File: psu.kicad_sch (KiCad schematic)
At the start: 63 parts, among them J3 USB_C_Receptacle_PowerOnly_24P, J4 Screw_Terminal_01x02, J5 Screw_Terminal_01x02, J6 Screw_Terminal_01x03, Q1 2N7002, Q2 DMP3099L, Q3 DMP3099L, U17 CYPD3177-24LQ, U19 LM2596S-ADJ, U20 INA180A3, U21 LM2596S-5, U22 LM2596S-5

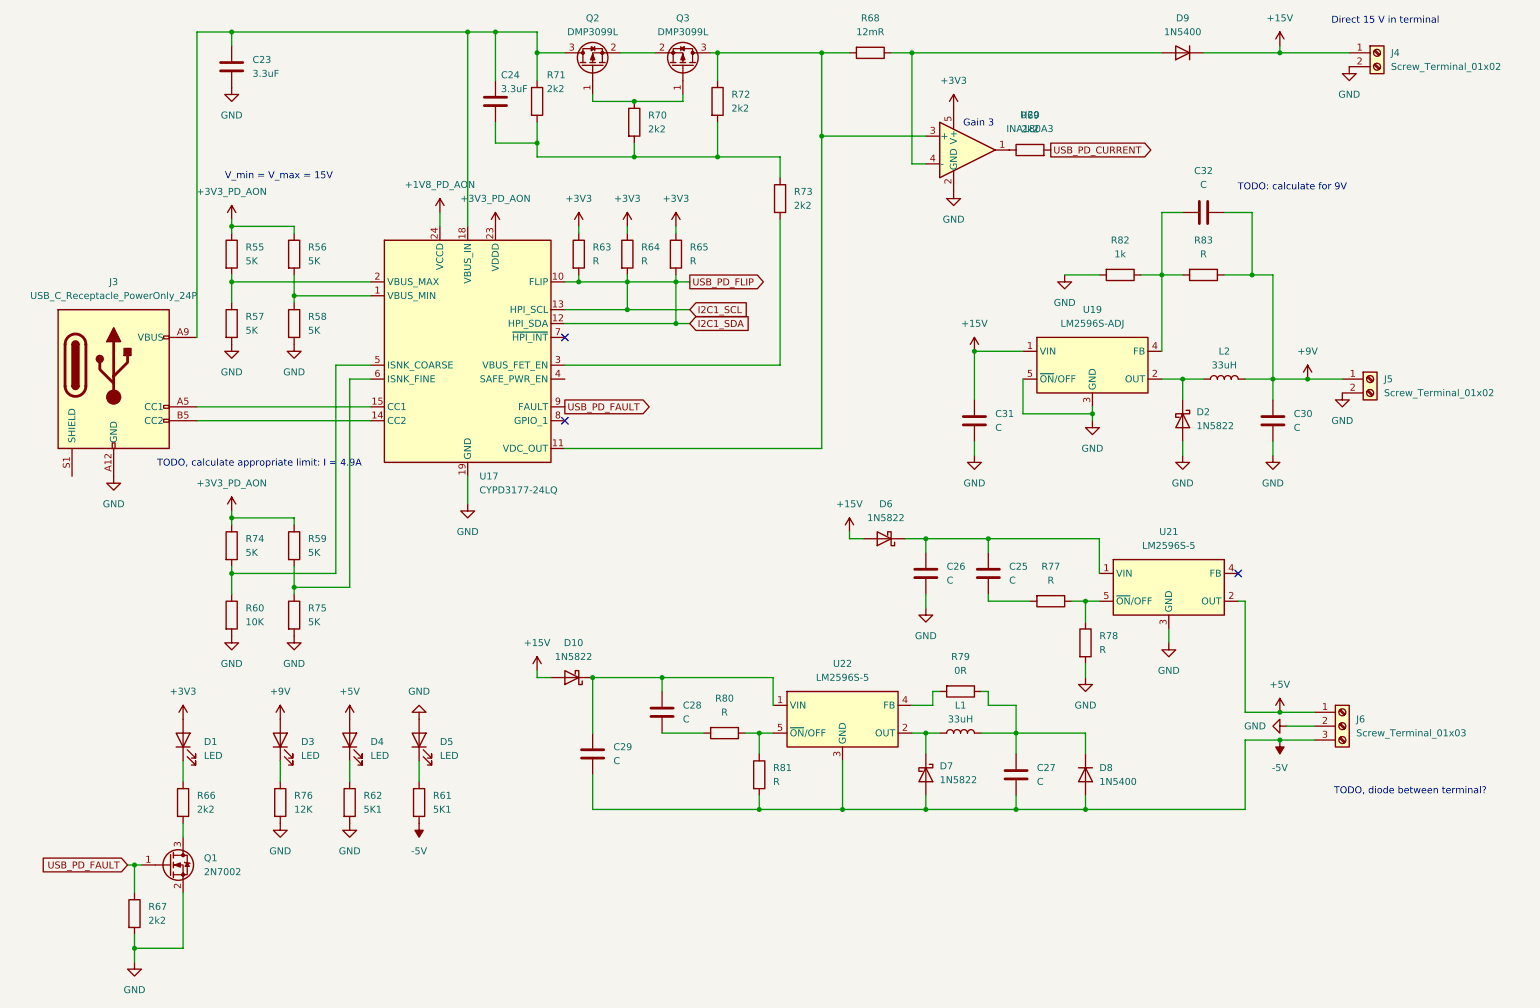
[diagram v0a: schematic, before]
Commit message: Save work on simplifying the desing
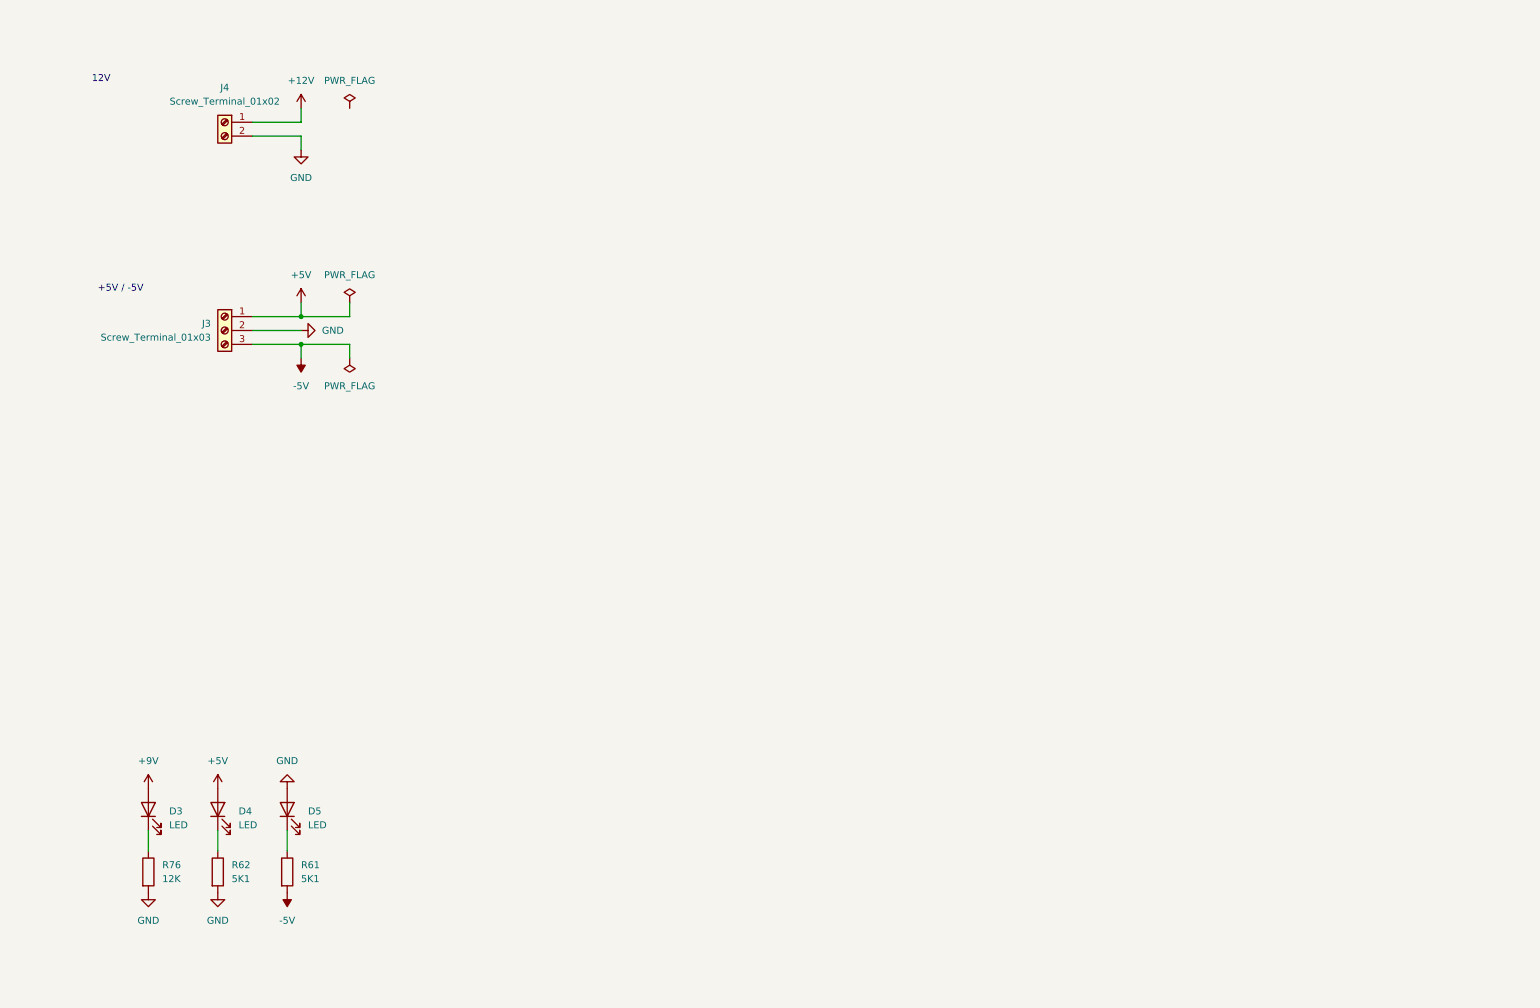
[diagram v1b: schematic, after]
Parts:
- removed C23, C24: 3.3uF, symbol Device:C
- removed C25, C26, C27, C28, C29, C30, C31, C32: C, symbol Device:C
- removed D1: LED, symbol Device:LED
- removed D10, D2, D6, D7: 1N5822, Diode_THT:D_DO-201AD_P15.24mm_Horizontal, symbol Diode:1N5822
- removed D8, D9: 1N5400, Diode_THT:D_DO-201AD_P15.24mm_Horizontal, symbol Diode:1N5400
- removed J3: USB_C_Receptacle_PowerOnly_24P, symbol Connector:USB_C_Receptacle_PowerOnly_24P
- removed J5: Screw_Terminal_01x02, symbol Connector:Screw_Terminal_01x02
- removed J6: Screw_Terminal_01x03, symbol Connector:Screw_Terminal_01x03
- removed L1, L2: 33uH, symbol Device:L
- removed Q1: 2N7002, Package_TO_SOT_SMD:SOT-23, symbol Transistor_FET:2N7002
- removed Q2, Q3: DMP3099L, Package_TO_SOT_SMD:SOT-23, symbol Transistor_FET:DMP3099L
- removed R55, R56, R57, R58, R59, R74, R75: 5K, symbol Device:R
- removed R60: 10K, symbol Device:R
- removed R63, R64, R65, R77, R78, R80, R81, R83: R, symbol Device:R
- removed R66, R67, R69, R70, R71, R72, R73: 2k2, symbol Device:R
- removed R68: 12mR, symbol Device:R
- removed R79: 0R, symbol Device:R
- removed R82: 1k, symbol Device:R
- removed U17: CYPD3177-24LQ, Package_DFN_QFN:QFN-24-1EP_4x4mm_P0.5mm_EP2.75x2.75mm, symbol Interface_USB:CYPD3177-24LQ
- removed U19: LM2596S-ADJ, Package_TO_SOT_SMD:TO-263-5_TabPin3, symbol Regulator_Switching:LM2596S-ADJ
- removed U20: INA180A3, Package_TO_SOT_SMD:SOT-23-5, symbol Amplifier_Current:INA180A3
- removed U21, U22: LM2596S-5, Package_TO_SOT_SMD:TO-263-5_TabPin3, symbol Regulator_Switching:LM2596S-5
- added J3: Screw_Terminal_01x03, symbol Connector:Screw_Terminal_01x03
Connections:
- net +5V: now also J3.1 (Pin_1)
- net -5V: now also J3.3 (Pin_3)
- net GND: now also J3.2 (Pin_2)
- net +15V renamed +12V
- no-connect marks 3 -> 0
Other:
- note added: "+5V / -5V"
- note added: "12V"
- note removed: "Direct 15 V in terminal"
- note removed: "Gain 3"
- note removed: "TODO, calculate appropriate limit: I = 4.9A"
- note removed: "TODO, diode between terminal?"
- note removed: "TODO: calculate for 9V"
- note removed: "V_min = V_max = 15V"
- moved on the sheet: D3, D4, D5, R61, R62, R76
